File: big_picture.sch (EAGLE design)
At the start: 10 parts, among them K1 RELAY-SPDT-JZC-11F, M1 MOTOR10MM

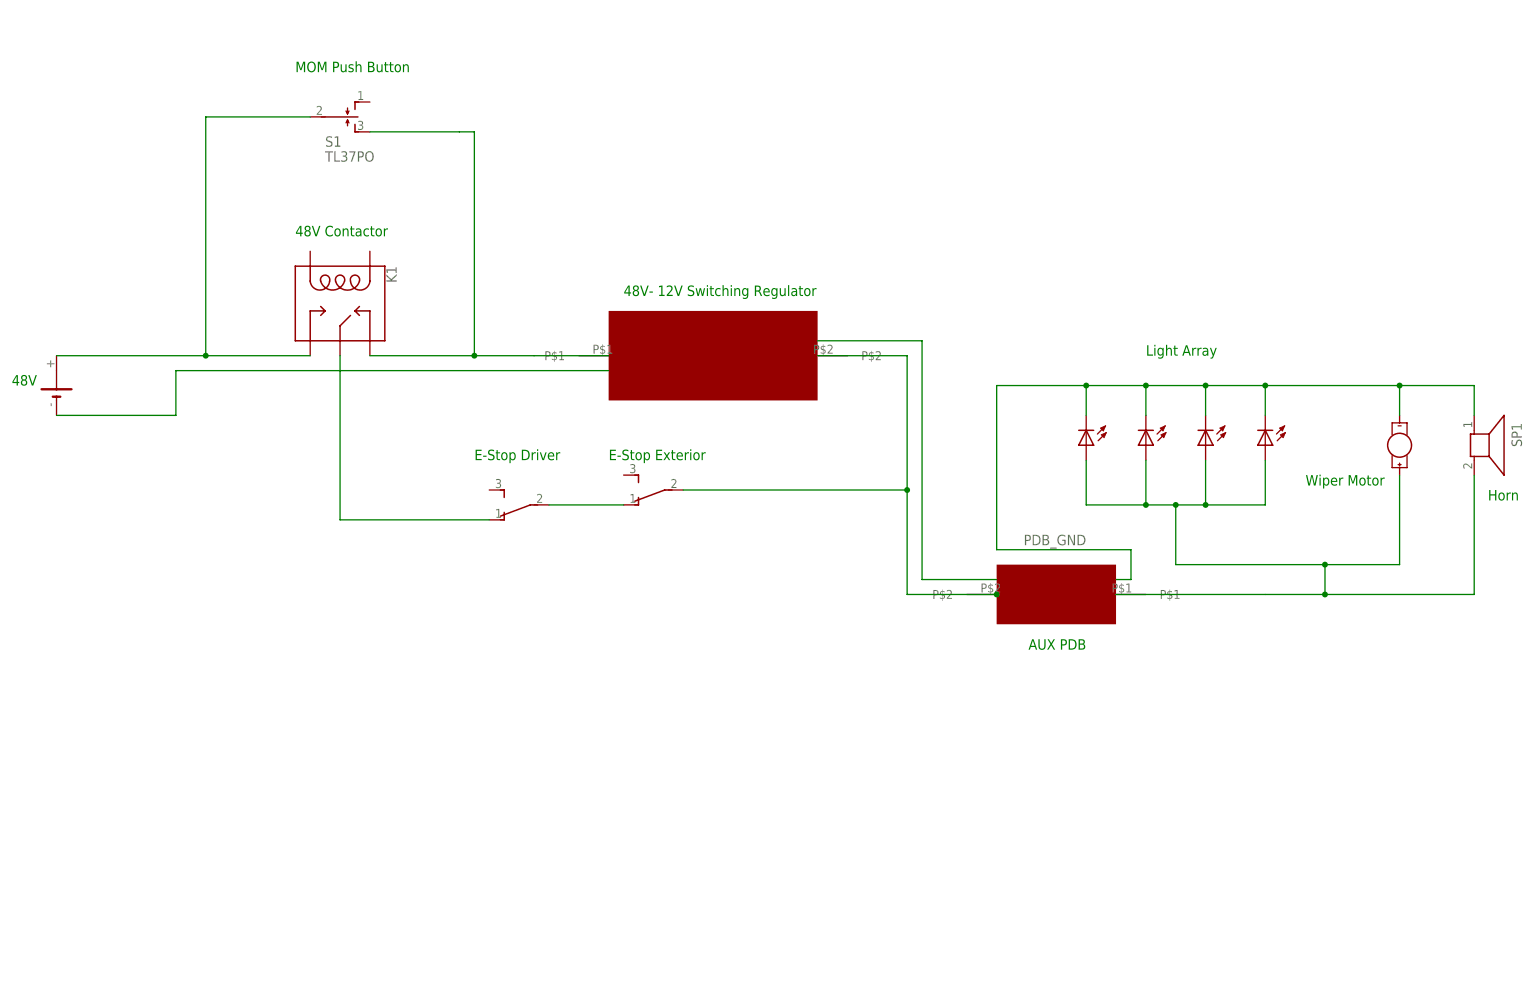
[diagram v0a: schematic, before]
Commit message: redid general schematic
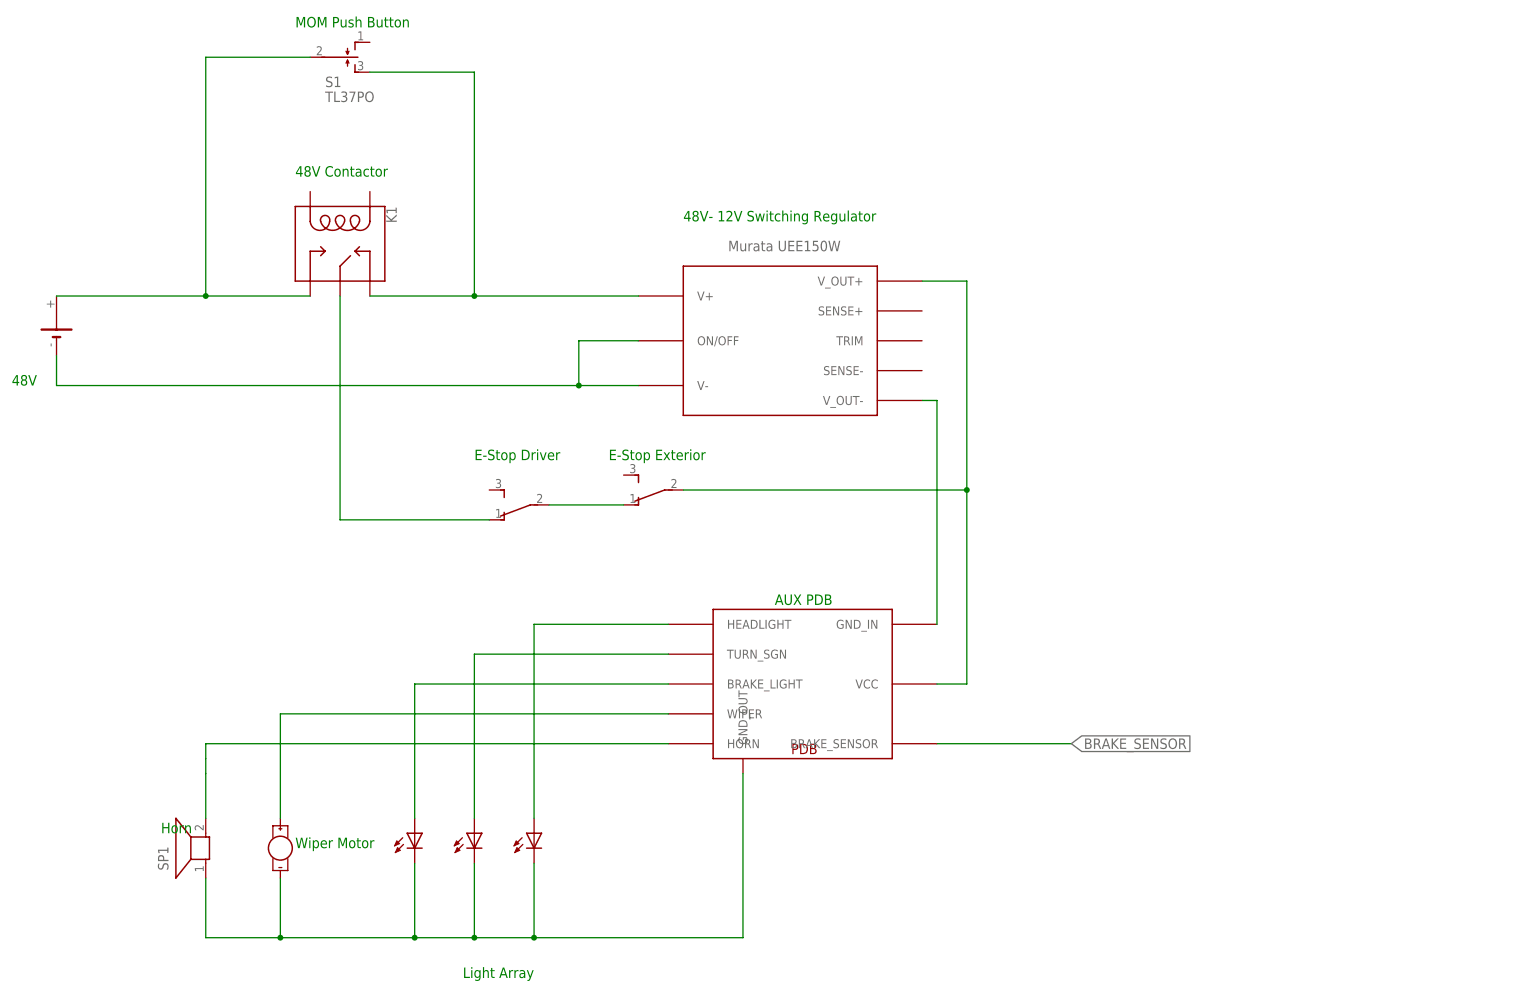
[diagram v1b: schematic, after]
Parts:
- U$4: value BUCK -> UEE150W; device big_picture_parts:BUCK -> REV Aux Circuit:UEE150W
- U$5: value AUX -> PDB_OUTLINE; device big_picture_parts:AUX -> REV Aux Circuit:PDB_OUTLINE
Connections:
- new net BRAKE_SENSOR: U$5.BRAKE_SENSOR
- new net N$10: U$4.V_OUT-, U$5.GND_IN
- new net N$4: G1.-, U$4.ON/OFF, U$4.V-
- new net N$8: DZ1-3.A, U$5.HEADLIGHT
- new net N$9: DZ1-2.A, U$5.TURN_SGN
- net N$1: now also U$4.V_OUT+, U$5.VCC; no longer U$4.P$2
- net N$2: now also DZ1-1.A, U$5.BRAKE_LIGHT; no longer G1.-
- net N$31: now also U$5.HORN; no longer DZ1-1.A, DZ1-2.A, DZ1-3.A, DZ1-4.A, M1.+, U$5.P$1
- net N$35: now also U$4.V+; no longer U$4.P$1
- net N$5: now also M1.+, U$5.WIPER; no longer U$5.P$2
- net PDB_GND: now also U$5.GND_OUT; no longer DZ1-4.C
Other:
- moved on the sheet: K1, S1, SP1
